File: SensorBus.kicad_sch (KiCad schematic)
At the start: 6 parts, among them U1 BNO055_IC2, U302 TFmini_S Lidar, U303 TFmini_S Lidar, U304 TFmini_S Lidar

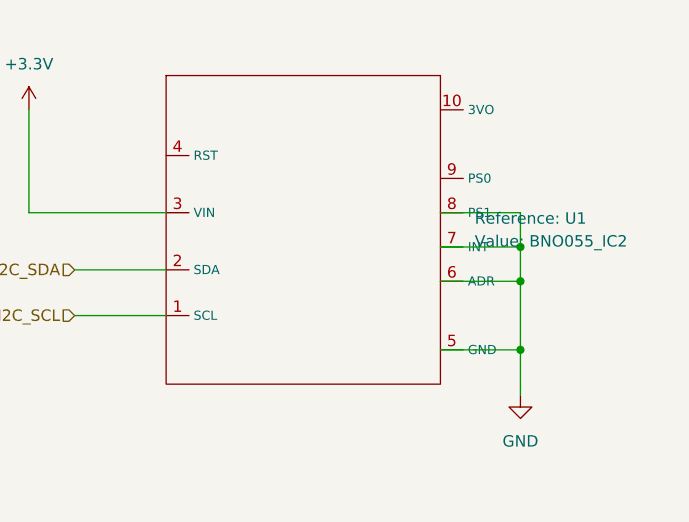
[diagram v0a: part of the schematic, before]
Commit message: changed one thing
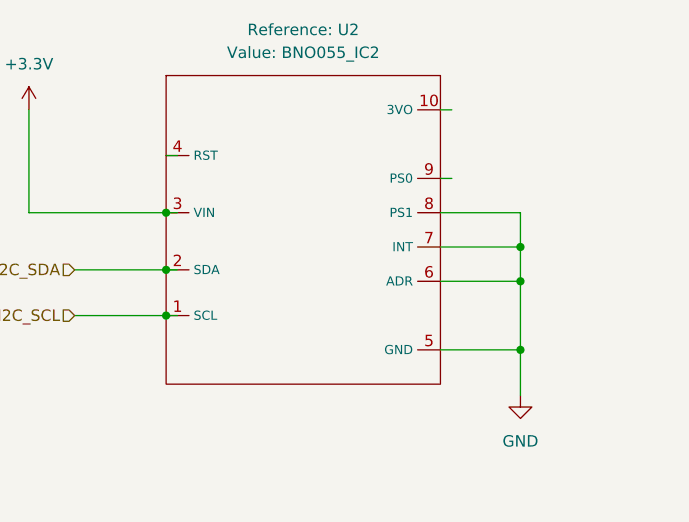
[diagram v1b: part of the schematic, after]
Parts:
- removed U1: BNO055_IC2, symbol sensors5:BNO055_IC2
- added U2: BNO055_IC2, symbol sensors2:BNO055_IC2
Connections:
- net +3.3V: now also U2.3 (VIN)
- net GND: now also U2.5 (GND), U2.6 (ADR), U2.7 (INT), U2.8 (PS1)
- net I2C_SCL: now also U2.1 (SCL)
- net I2C_SDA: now also U2.2 (SDA)
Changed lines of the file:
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@@
+	)
+	(junction
+		(at 208.28 71.12)
+		(diameter 0)
+		(color 0 0 0 0)
 	)
 	(junction
@@
 	)
 	(junction
+		(at 208.28 59.69)
+		(diameter 0)
+		(color 0 0 0 0)
+	)
+	(junction
 		(at 247.65 67.31)
 		(diameter 0)
 		(color 0 0 0 0)
 	)
+	(junction
+		(at 208.28 66.04)
+		(diameter 0)
+		(color 0 0 0 0)
+	)
+	(wire
+		(pts
+			(xy 209.55 53.34) (xy 208.28 53.34)
+		)
+		(stroke
+			(width 0)
+			(type default)
+		)
+	)
 	(wire
 		(pts
@@
 	(wire
 		(pts
+			(xy 209.55 71.12) (xy 208.28 71.12)
+		)
+		(stroke
+			(width 0)
+			(type default)
+		)
+	)
+	(wire
+		(pts
 			(xy 97.79 168.91) (xy 101.6 168.91)
 		)
@@
 	(wire
 		(pts
+			(xy 209.55 66.04) (xy 208.28 66.04)
+		)
+		(stroke
+			(width 0)
+			(type default)
+		)
+	)
+	(wire
+		(pts
 			(xy 95.25 130.81) (xy 100.33 130.81)
 		)
@@
 	(wire
 		(pts
+			(xy 240.03 48.26) (xy 238.76 48.26)
+		)
+		(stroke
+			(width 0)
+			(type default)
+		)
+	)
+	(wire
+		(pts
 			(xy 247.65 63.5) (xy 247.65 67.31)
 		)
@@
 	(wire
 		(pts
+			(xy 209.55 59.69) (xy 208.28 59.69)
+		)
+		(stroke
+			(width 0)
+			(type default)
+		)
+	)
+	(wire
+		(pts
 			(xy 238.76 63.5) (xy 247.65 63.5)
 		)
@@
 	(wire
 		(pts
+			(xy 91.44 97.79) (xy 102.87 97.79)
+		)
+		(stroke
+			(width 0)
+			(type default)
+		)
+	)
+	(wire
+		(pts
+			(xy 90.17 153.67) (xy 101.6 153.67)
+		)
+		(stroke
+			(width 0)
+			(type default)
+		)
+	)
+	(wire
+		(pts
+			(xy 166.37 97.79) (xy 163.83 97.79)
+		)
+		(stroke
+			(width 0)
+			(type default)
+		)
+	)
+	(wire
+		(pts
+			(xy 96.52 135.89) (xy 100.33 135.89)
+		)
+		(stroke
+			(width 0)
+			(type default)
+		)
+	)
+	(wire
+		(pts
+			(xy 99.06 107.95) (xy 102.87 107.95)
+		)
+		(stroke
+			(width 0)
+			(type default)
+		)
+	)
+	(wire
+		(pts
 			(xy 238.76 59.69) (xy 247.65 59.69)
 		)
@@
 	(wire
 		(pts
-			(xy 91.44 97.79) (xy 102.87 97.79)
-		)
-		(stroke
-			(width 0)
-			(type default)
-		)
-	)
-	(wire
-		(pts
-			(xy 90.17 153.67) (xy 101.6 153.67)
-		)
-		(stroke
-			(width 0)
-			(type default)
-		)
-	)
-	(wire
-		(pts
-			(xy 166.37 97.79) (xy 163.83 97.79)
-		)
-		(stroke
-			(width 0)
-			(type default)
-		)
-	)
-	(wire
-		(pts
-			(xy 96.52 135.89) (xy 100.33 135.89)
-		)
-		(stroke
-			(width 0)
-			(type default)
-		)
-	)
-	(wire
-		(pts
-			(xy 99.06 107.95) (xy 102.87 107.95)
-		)
-		(stroke
-			(width 0)
-			(type default)
-		)
-	)
-	(wire
-		(pts
 			(xy 193.04 59.69) (xy 208.28 59.69)
 		)
@@
 		(pts
 			(xy 198.12 71.12) (xy 208.28 71.12)
+		)
+		(stroke
+			(width 0)
+			(type default)
+		)
+	)
+	(wire
+		(pts
+			(xy 240.03 55.88) (xy 238.76 55.88)
 		)
 		(stroke
@@
 				(path "/241fe27d-f15c-49f2-a703-528239fb7ddd/47a17038-38f9-4ccd-a989-e4987ae8c367"
 					(reference "R302")
-					(unit 1)
-				)
-			)
-		)
-	)
-	(symbol
-		(lib_id "sensors5:BNO055_IC2")
-		(at 223.52 41.91 0)
-		(unit 1)
-		(exclude_from_sim no)
-		(in_bom yes)
-		(on_board yes)
-		(dnp no)
-		(fields_autoplaced yes)
-		(property "Reference" "U1"
-			(at 242.57 60.3249 0)
-			(show_name yes)
-			(effects
-				(font
-					(size 1.27 1.27)
-				)
-				(justify left)
-			)
-		)
-		(property "Value" "BNO055_IC2"
-			(at 242.57 62.8649 0)
-			(show_name yes)
-			(effects
-				(font
-					(size 1.27 1.27)
-				)
-				(justify left)
-			)
-		)
-		(property "Footprint" ""
-			(at 223.52 41.91 0)
-			(effects
-				(font
-					(size 1.27 1.27)
-				)
-				(hide yes)
-			)
-		)
-		(property "Datasheet" ""
-			(at 223.52 41.91 0)
-			(effects
-				(font
-					(size 1.27 1.27)
-				)
-				(hide yes)
-			)
-		)
-		(property "Description" ""
-			(at 223.52 41.91 0)
-			(effects
-				(font
-					(size 1.27 1.27)
-				)
-				(hide yes)
-			)
-		)
-		(pin "8"
-		)
-		(pin "6"
-		)
-		(pin "5"
-		)
-		(pin "4"
-		)
-		(pin "3"
-		)
-		(pin "7"
-		)
-		(pin "2"
-		)
-		(pin "1"
-		)
-		(pin "9"
-		)
-		(pin "10"
-		)
-		(instances
-			(project ""
-				(path "/241fe27d-f15c-49f2-a703-528239fb7ddd/47a17038-38f9-4ccd-a989-e4987ae8c367"
-					(reference "U1")
 					(unit 1)
 				)
@@
 					(unit 1)
 				)
+			)
+		)
+	)
+	(symbol
+		(lib_id "sensors2:BNO055_IC2")
+		(at 223.52 41.91 0)
+		(unit 1)
+		(exclude_from_sim no)
+		(in_bom yes)
+		(on_board yes)
+		(dnp no)
+		(fields_autoplaced yes)
+		(property "Reference" "U2"
+			(at 223.52 39.37 0)
+			(show_name yes)
+			(effects
+				(font
+					(size 1.27 1.27)
+				)
+			)
+		)
+		(property "Value" "BNO055_IC2"
+			(at 223.52 41.91 0)
+			(show_name yes)
+			(effects
+				(font
+					(size 1.27 1.27)
+				)
+			)
+		)
+		(property "Footprint" ""
+			(at 223.52 41.91 0)
+			(effects
+				(font
+					(size 1.27 1.27)
+				)
+				(hide yes)
+			)
+		)
+		(property "Datasheet" ""
+			(at 223.52 41.91 0)
+			(effects
+				(font
+					(size 1.27 1.27)
+				)
+				(hide yes)
+			)
+		)
+		(property "Description" ""
+			(at 223.52 41.91 0)
+			(effects
+				(font
+					(size 1.27 1.27)
+				)
+				(hide yes)
+			)
+		)
+		(pin "3"
+		)
+		(pin "2"
+		)
+		(pin "1"
+		)
+		(pin "6"
+		)
+		(pin "7"
+		)
+		(pin "5"
+		)
+		(pin "4"
+		)
+		(pin "8"
+		)
+		(pin "9"
+		)
+		(pin "10"
+		)
+		(instances
+			(project ""
+				(path "/241fe27d-f15c-49f2-a703-528239fb7ddd/47a17038-38f9-4ccd-a989-e4987ae8c367"
+					(reference "U2")
+					(unit 1)
+				)
